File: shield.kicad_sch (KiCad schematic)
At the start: 5 parts, among them J1 Conn_01x20, J2 Conn_01x20

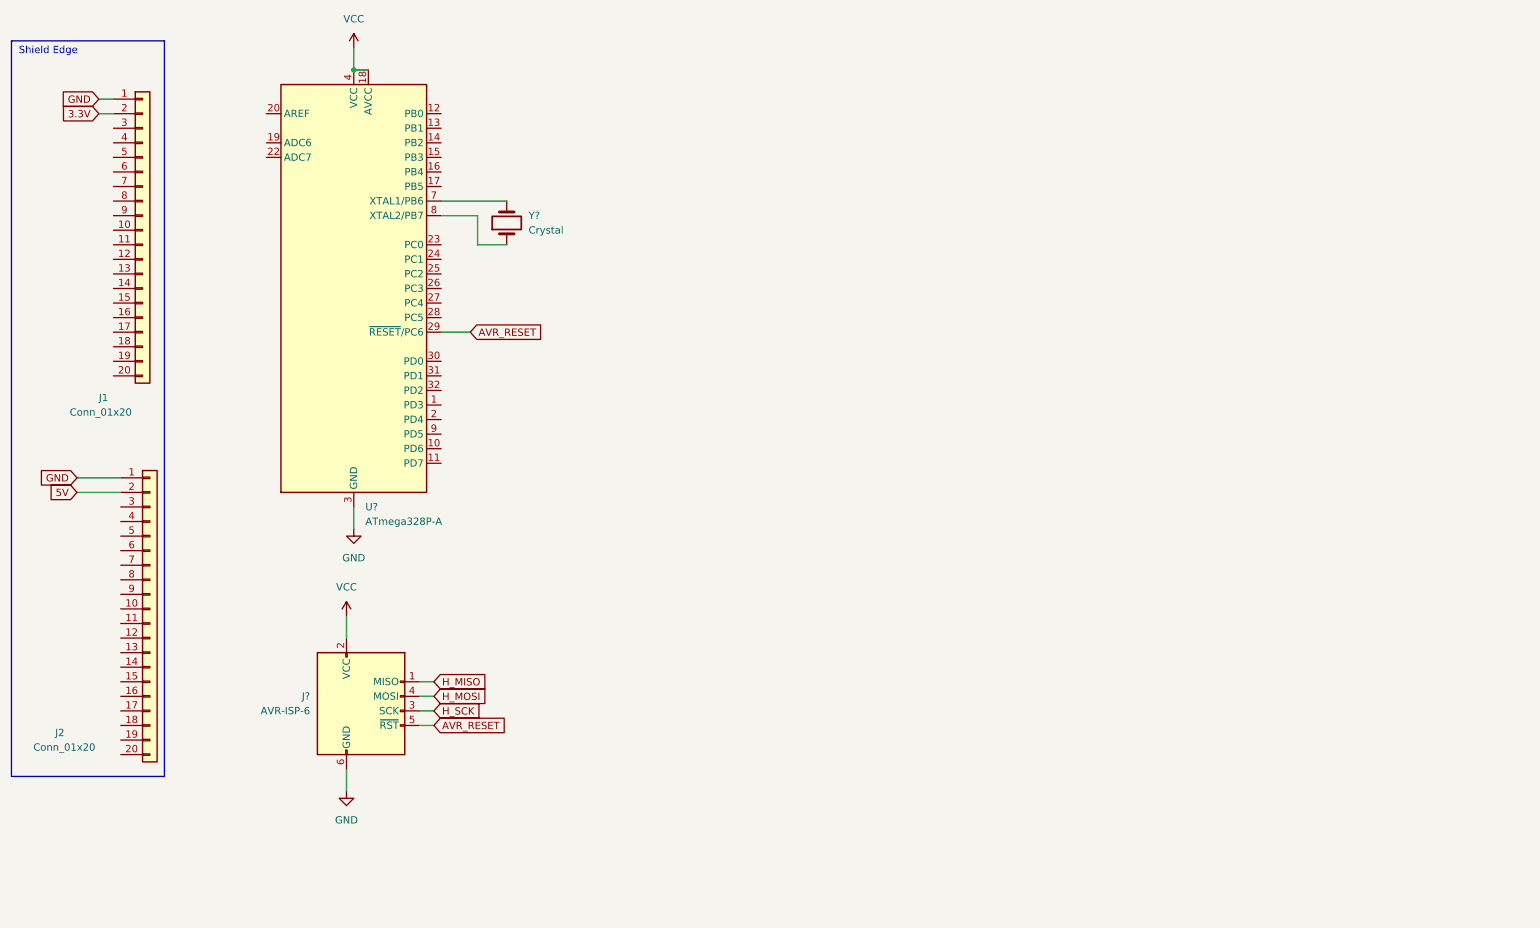
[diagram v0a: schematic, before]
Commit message: poop
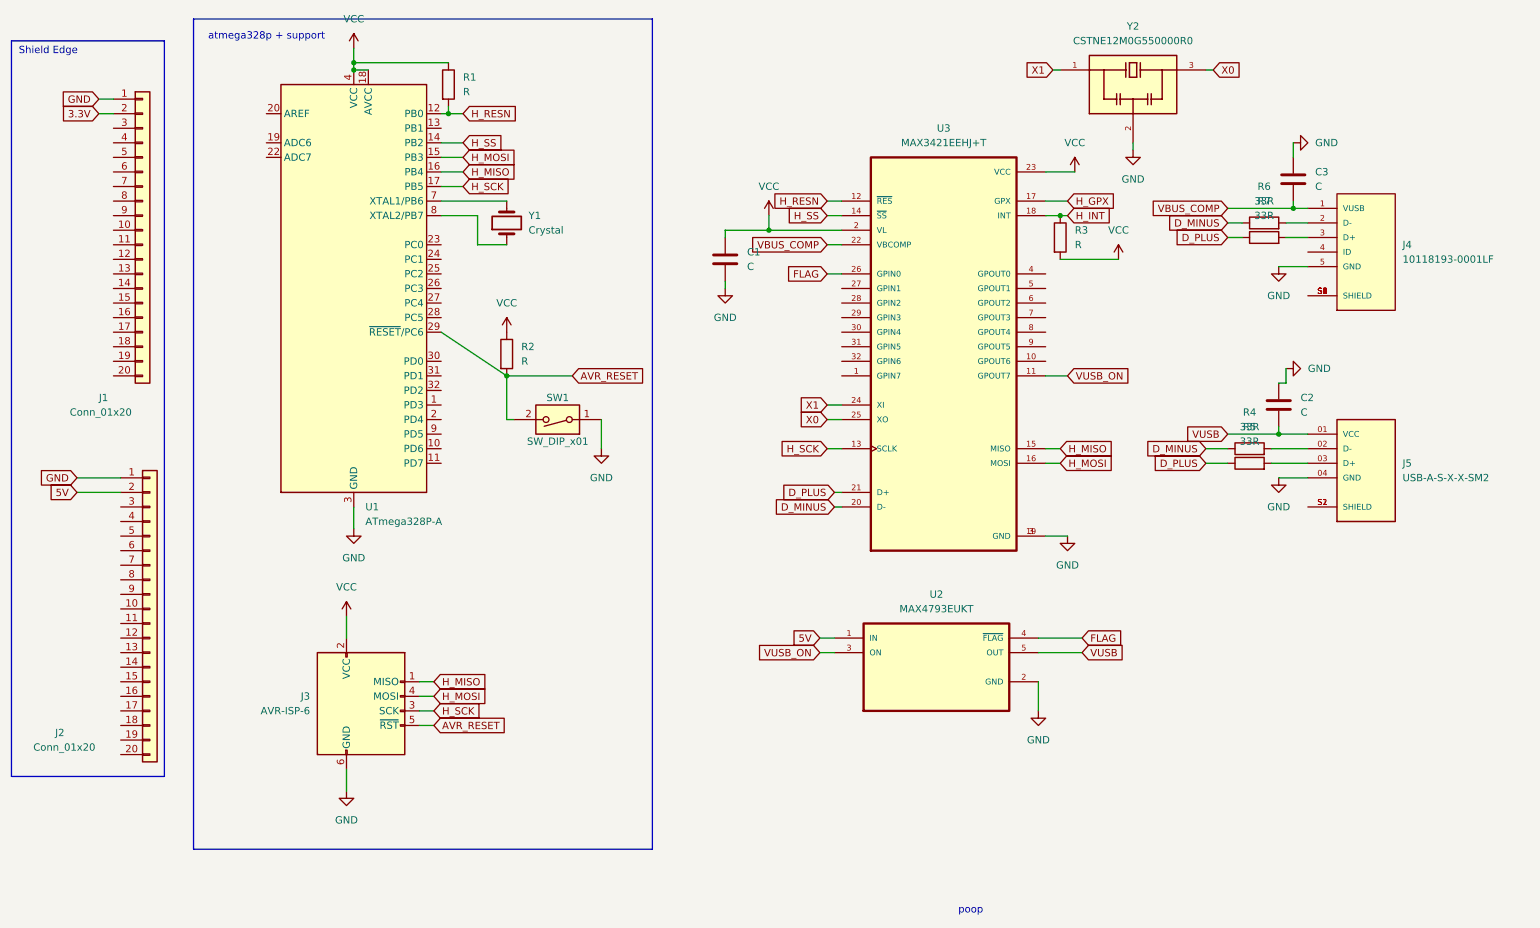
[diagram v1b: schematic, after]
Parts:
- added C1, C2, C3: C, symbol Device:C
- added J4: 10118193-0001LF, shield_rsrc:FCI_10118193-0001LF, symbol shield_rsrc:10118193-0001LF
- added J5: USB-A-S-X-X-SM2, shield_rsrc:SAMTEC_USB-A-S-X-X-SM2, symbol shield_rsrc:USB-A-S-X-X-SM2
- added R1, R2, R3: R, symbol Device:R
- added R4, R5, R6, R7: 33R, Resistor_SMD:R_0603_1608Metric_Pad0.98x0.95mm_HandSolder, symbol Device:R
- added SW1: SW_DIP_x01, symbol Switch:SW_DIP_x01
- added U2: MAX4793EUKT, shield_rsrc:SOT95P280X145-5N, symbol shield_rsrc:MAX4793EUKT
- added U3: MAX3421EEHJ+T, shield_rsrc:QFP50P700X700X120-32N, symbol shield_rsrc:MAX3421EEHJ+T
- added Y2: CSTNE12M0G550000R0, OSC_CSTNE12M0G550000R0, symbol shield_rsrc:CSTNE12M0G550000R0
- gave numbers to parts that had none: 3
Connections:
- net 5V: now also U2.1 (IN)
- net AVR_RESET: now also R2.2, SW1.2
- net GND: now also C1.2, C2.1, C3.1, J4.5 (GND), J5.04 (GND), SW1.1, U2.2 (GND), U3.19 (GND), U3.3 (GND), Y2.2
- net H_MISO: now also U1.16 (PB4), U3.15 (MISO)
- net H_MOSI: now also U1.15 (PB3), U3.16 (MOSI)
- net H_SCK: now also U1.17 (PB5), U3.13 (SCLK)
- net VCC: now also C1.1, R1.1, R2.1, R3.2, U3.2 (VL), U3.23 (VCC)
- net H_RESN: now reaches U1.12 (PB0)
- net H_RESN: now also R1.2, U3.12 (~{RES})
- net H_SS: now reaches U1.14 (PB2)
- net H_SS: now also U3.14 (~{SS})
- new net: J5.03 (D+), R5.2
- new net: J4.2 (D-), R6.2
- new net: J4.3 (D+), R7.2
- new net: J4.S1 (SHIELD), J4.S2 (SHIELD), J4.S3 (SHIELD), J4.S4 (SHIELD), J4.S5 (SHIELD), J4.S6 (SHIELD)
- new net: J5.02 (D-), R4.2
- new net: J5.S1 (SHIELD), J5.S2 (SHIELD)
- new net D_MINUS: R4.1, R6.1, U3.20 (D-)
- new net D_PLUS: R5.1, R7.1, U3.21 (D+)
- new net FLAG: U2.4 (~{FLAG}), U3.26 (GPIN0)
- new net H_GPX: U3.17 (GPX)
- new net H_INT: R3.1, U3.18 (INT)
- new net VBUS_COMP: C3.2, J4.1 (VUSB), U3.22 (VBCOMP)
- new net VUSB: C2.2, J5.01 (VCC), U2.5 (OUT)
- new net VUSB_ON: U2.3 (ON), U3.11 (GPOUT7)
- new net X0: U3.25 (XO), Y2.3
- new net X1: U3.24 (XI), Y2.1
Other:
- note added: "atmega328p + support"
- note added: "poop"
